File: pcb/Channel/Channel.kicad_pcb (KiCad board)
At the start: 2 copper layers, 44 x 196 mm, 11 parts, among them J1 Mainboard, J2 SPI_CHAIN_IN, J3 SPI_CHAIN_OUT, J4 Motor_Out, J6 Motor_In, SW1 RotaryEncoder_Switch

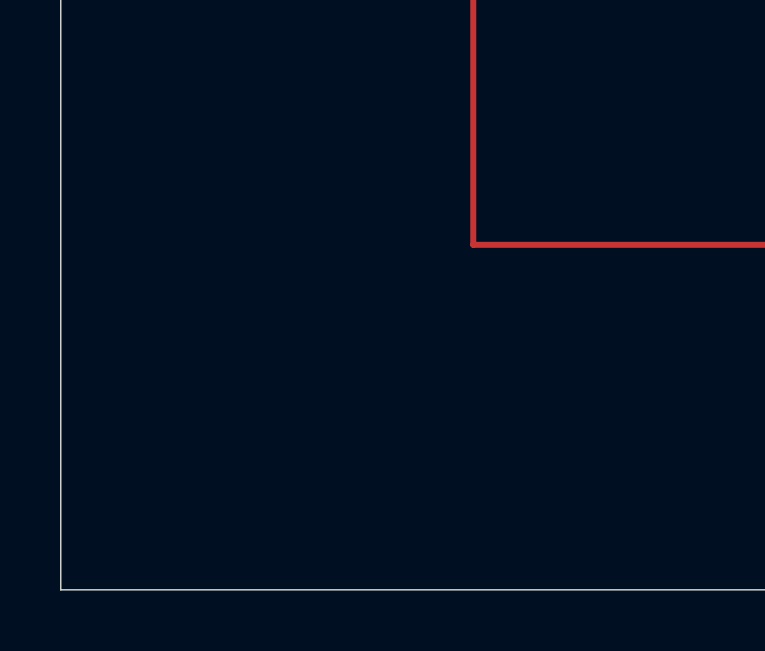
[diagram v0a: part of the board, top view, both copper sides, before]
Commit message: Silkscreen updates.
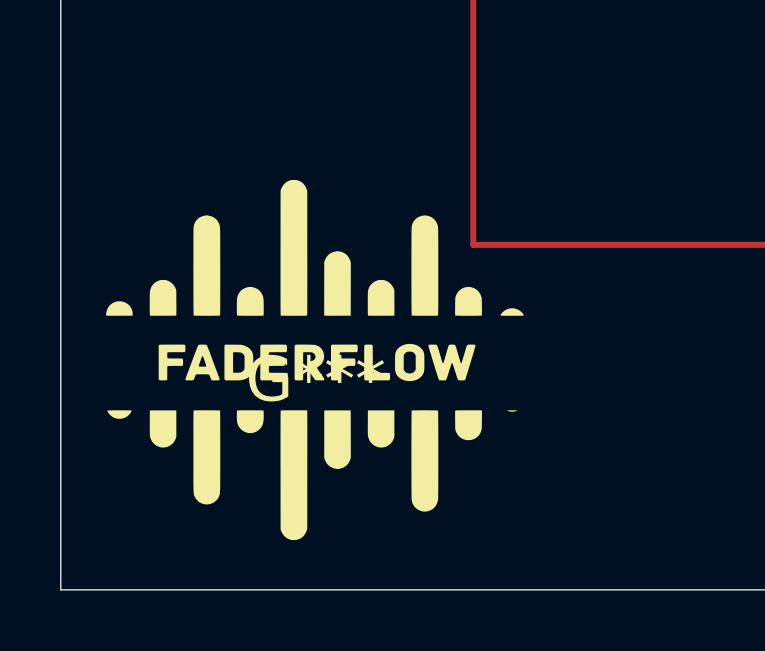
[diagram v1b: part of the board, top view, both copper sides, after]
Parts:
- added G***: LOGO, LOGO, F.Cu at (53.5, 233.0)

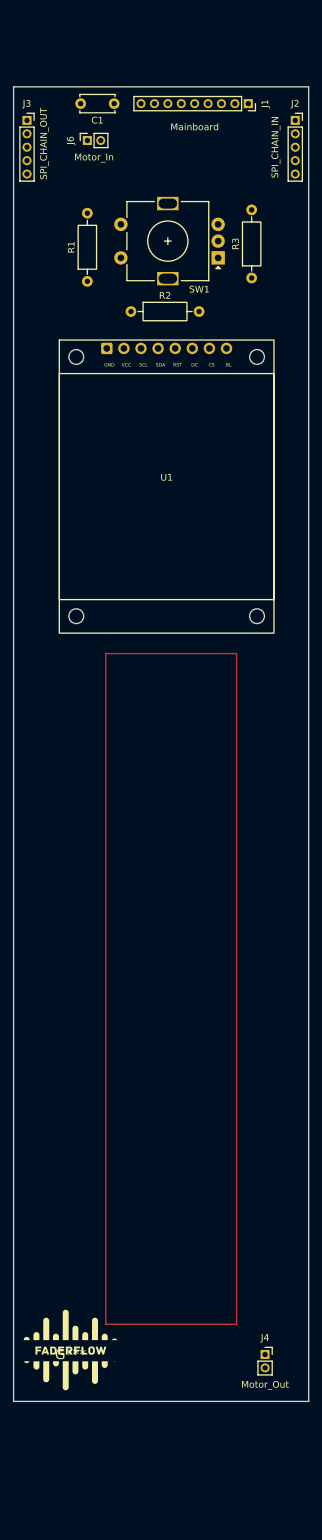
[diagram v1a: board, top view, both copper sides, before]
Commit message: Fix up channel pcb
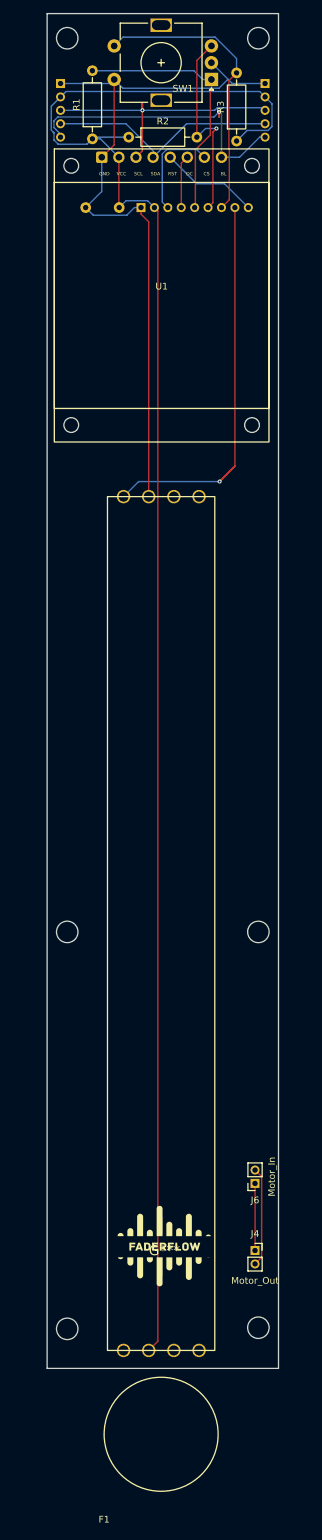
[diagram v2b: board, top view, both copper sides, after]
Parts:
- added F1: ~, Behringer X32 Fader:Behringer X32 Fader, F.Cu at (59.0, 98.6)
- added Mount_1: MountingHole_3.2mm_M3, MountingHole:MountingHole_3.2mm_M3, F.Cu at (53.0, 36.8)
- added Mount_2: MountingHole_3.2mm_M3, MountingHole:MountingHole_3.2mm_M3, F.Cu at (81.5, 36.8)
- added Mount_3: MountingHole_3.2mm_M3, MountingHole:MountingHole_3.2mm_M3, F.Cu at (53.0, 170.0)
- added Mount_4: MountingHole_3.2mm_M3, MountingHole:MountingHole_3.2mm_M3, F.Cu at (81.5, 170.0)
- added Mount_6: MountingHole_3.2mm_M3, MountingHole:MountingHole_3.2mm_M3, F.Cu at (53.0, 229.2)
- added Mount_7: MountingHole_3.2mm_M3, MountingHole:MountingHole_3.2mm_M3, F.Cu at (81.5, 229.0)
- C1, J1, J2, J3: moved to B.Cu
- moved J6 157.5 mm to (81.0, 207.5), turned to 180 degrees
- moved U1 28.5 mm to (51.1, 53.2)
- moved SW1 26.6 mm to (74.5, 42.9)
- moved R2 26.0 mm to (62.2, 51.5)
- moved J1 22.3 mm to (64.0, 62.0)
- moved R1 21.3 mm to (56.8, 51.8)
- moved G*** 20.9 mm to (67.5, 217.5)
- moved R3 20.5 mm to (78.2, 52.1)
- moved C1 16.1 mm to (55.8, 62.0), turned to 0 degrees
- moved J4 15.6 mm to (81.0, 217.5)
- moved J3 7.43 mm to (52.0, 43.5), turned to 180 degrees
- moved J2 7.11 mm to (82.5, 43.5), turned to 180 degrees
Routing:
- net E_VCC: track 0.00 -> 251.3 mm
- net GND: track 0.00 -> 109.2 mm
- net FADER_OUT: track 0.00 -> 69.9 mm, vias 0 -> 1
- net SCR_BL_PWM: track 0.00 -> 45.8 mm, vias 0 -> 1
- net ENC_SW: track 0.00 -> 43.3 mm
- net SPI_SCK: track 0.00 -> 42.8 mm, vias 0 -> 1
- net ENC_CLK: track 0.00 -> 38.4 mm
- net SPI_MOSI: track 0.00 -> 34.9 mm
- net ENC_DT: track 0.00 -> 31.9 mm, vias 0 -> 1
- net SCREEN_CS: track 0.00 -> 15.4 mm
- net MOTOR-: track 0.00 -> 14.8 mm
- net SCREEN_RST: track 0.00 -> 14.8 mm
- net MOTOR+: track 0.00 -> 10.0 mm
- net SCREEN_DC: track 0.00 -> 7.87 mm
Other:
- board size 44 x 196 mm -> 34.5 x 202 mm
